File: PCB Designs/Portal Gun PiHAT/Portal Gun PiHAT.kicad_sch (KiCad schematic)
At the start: 26 parts, among them J1 GPIO, J2 SPARE_OUT_1, J3 SPARE_OUT_2, J4 NeoPixelFWD, J5 NeoPixelAFT, J6 5V Input, J7 PushButton2, J8 PushButton1, SW1 GPIO_SPARE_SW1, SW2 GPIO_SPARE_SW2, SW3 LED_PWR_SW, U1 CAT24C256

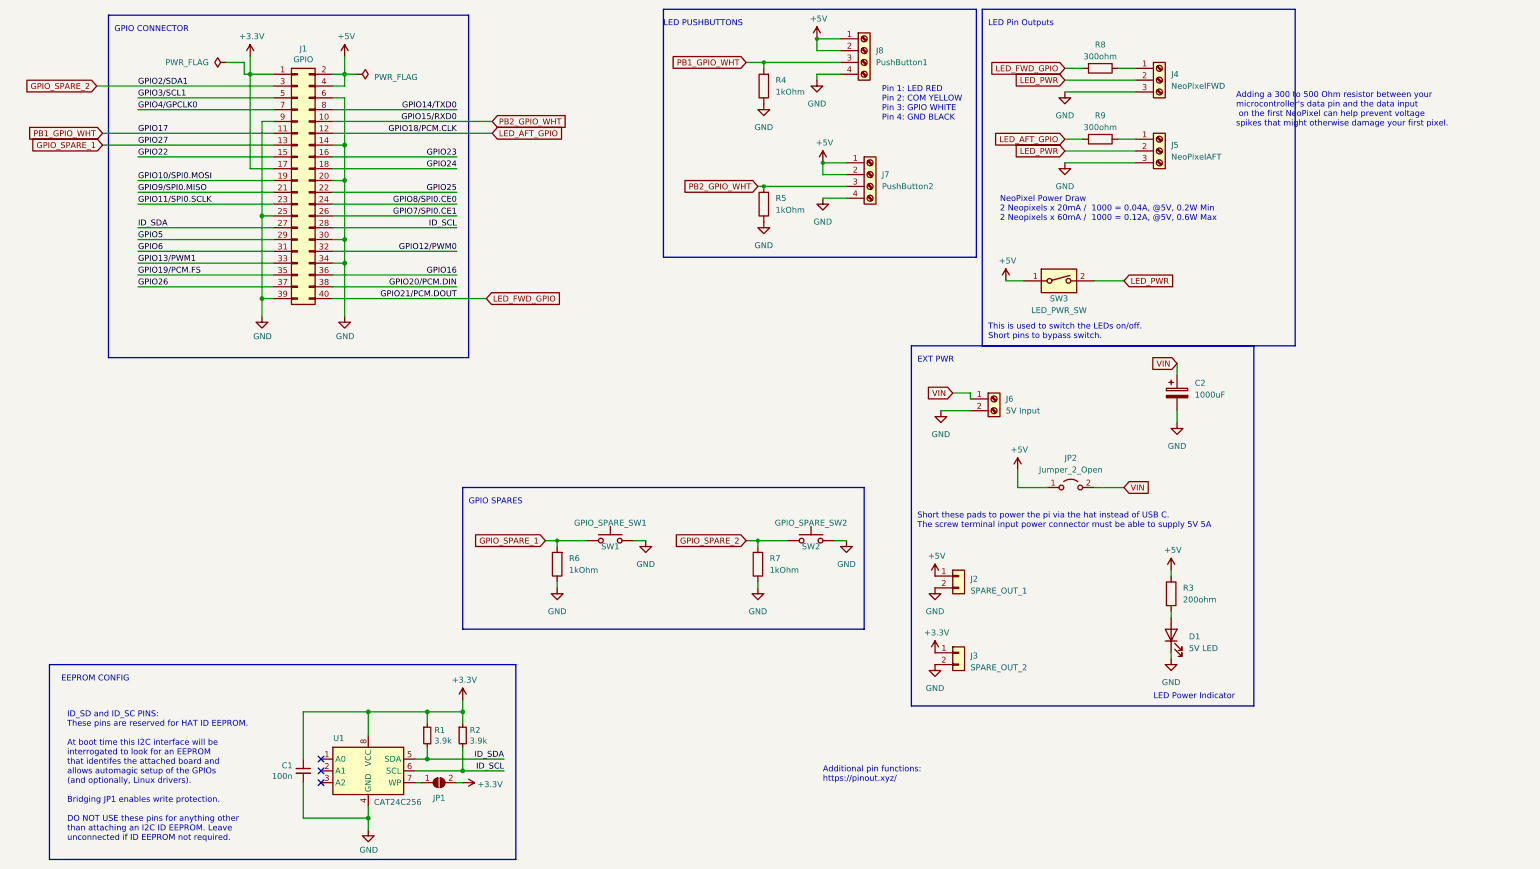
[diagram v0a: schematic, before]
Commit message: KiCad PCBs Finalized
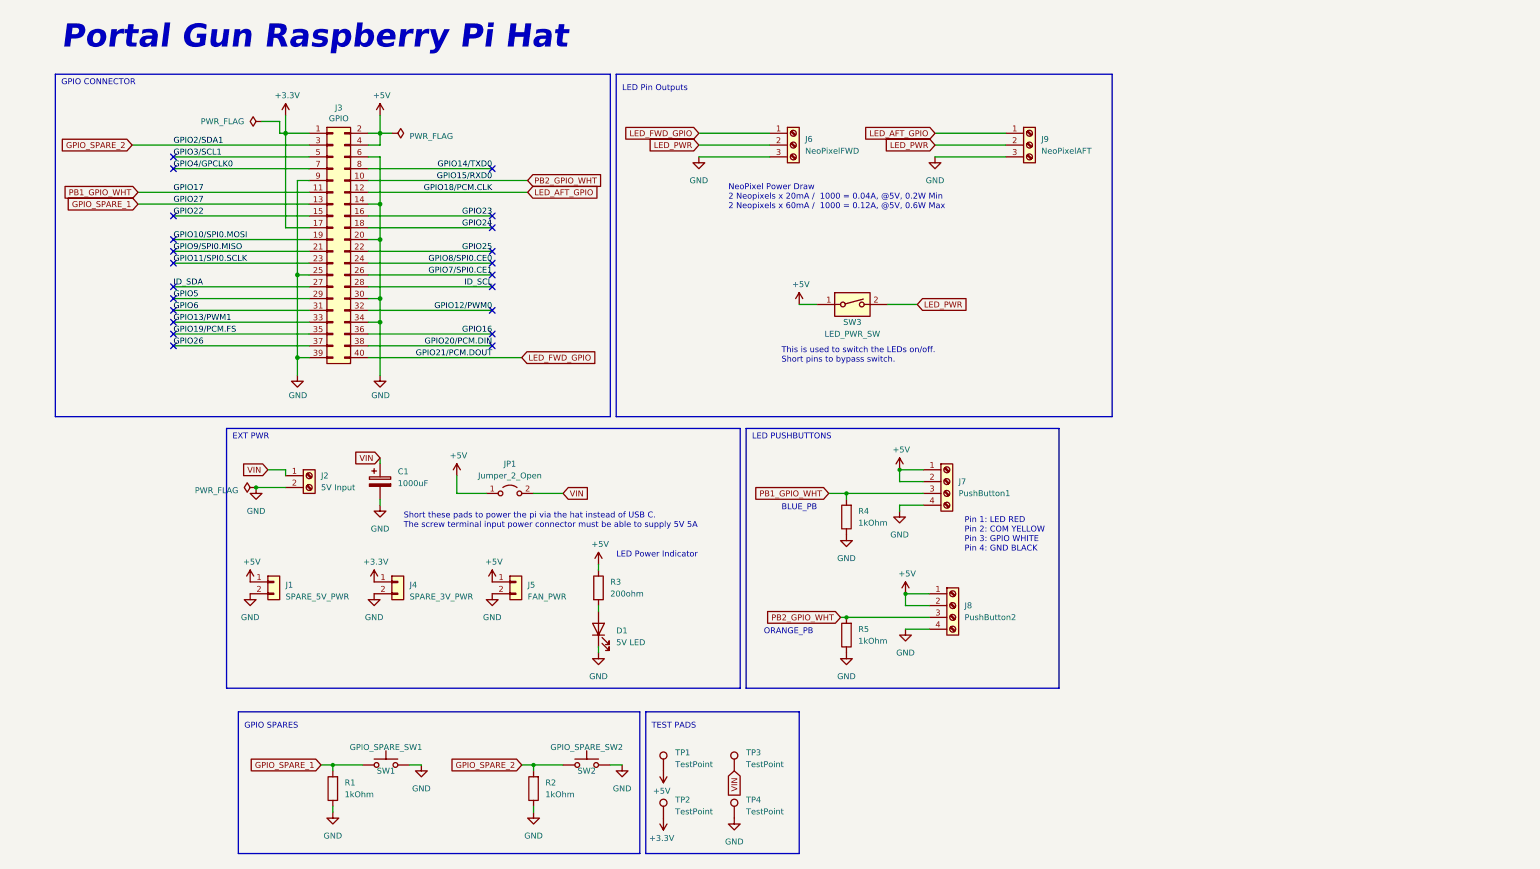
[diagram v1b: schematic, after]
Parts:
- removed C1: 100n, symbol Device:C_Small
- removed JP1: ID_WP, symbol Jumper:SolderJumper_2_Open
- removed R1, R2: 3.9k, symbol Device:R_Small
- removed R8, R9: 300ohm, symbol Device:R
- removed U1: CAT24C256, symbol Memory_EEPROM:CAT24C256
- added J5: FAN_PWR, Connector_PinHeader_2.54mm:PinHeader_1x02_P2.54mm_Vertical, symbol Connector_Generic:Conn_01x02
- added TP1, TP2, TP3, TP4: TestPoint, TestPoint:TestPoint_Pad_D1.0mm, symbol Connector:TestPoint
- C1: renamed from C2; footprint GrayFoxComponents:Horizontal Capacitor -> Capacitor_THT:C_Radial_D10.0mm_H16.0mm_P5.00mm
- D1: footprint (none) -> LED_THT:LED_D3.0mm
- J1: renamed from J2; value SPARE_OUT_1 -> SPARE_5V_PWR; footprint TerminalBlock_Phoenix:TerminalBlock_Phoenix_MKDS-1,5-2_1x02_P5.00mm_Horizontal -> Connector_PinHeader_2.54mm:PinHeader_1x02_P2.54mm_Vertical
- J2: renamed from J6; footprint (none) -> TerminalBlock_Phoenix:TerminalBlock_Phoenix_MKDS-1,5-2_1x02_P5.00mm_Horizontal
- J4: renamed from J3; value SPARE_OUT_2 -> SPARE_3V_PWR; footprint TerminalBlock_Phoenix:TerminalBlock_Phoenix_MKDS-1,5-2_1x02_P5.00mm_Horizontal -> Connector_PinHeader_2.54mm:PinHeader_1x02_P2.54mm_Vertical
- J6: renamed from J4; footprint (none) -> TerminalBlock_Phoenix:TerminalBlock_Phoenix_MKDS-1,5-3_1x03_P5.00mm_Horizontal
- J7: renamed from J8; footprint (none) -> TerminalBlock_Phoenix:TerminalBlock_Phoenix_MKDS-1,5-4_1x04_P5.00mm_Horizontal
- J8: renamed from J7; footprint (none) -> TerminalBlock_Phoenix:TerminalBlock_Phoenix_MKDS-1,5-4_1x04_P5.00mm_Horizontal
- J9: renamed from J5; footprint (none) -> TerminalBlock_Phoenix:TerminalBlock_Phoenix_MKDS-1,5-3_1x03_P5.00mm_Horizontal
- JP1: renamed from JP2; footprint (none) -> Jumper:SolderJumper-2_P1.3mm_Open_Pad1.0x1.5mm
- R1: renamed from R6; footprint (none) -> Resistor_SMD:R_1206_3216Metric_Pad1.30x1.75mm_HandSolder
- R2: renamed from R7; footprint (none) -> Resistor_SMD:R_1206_3216Metric_Pad1.30x1.75mm_HandSolder
- R3, R4, R5: footprint (none) -> Resistor_SMD:R_1206_3216Metric_Pad1.30x1.75mm_HandSolder
- renumbered J1 to J3
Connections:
- net +3V3: now also TP2.1
- net +5V: now also J5.1 (Pin_1), TP1.1
- net GND: now also J5.2 (Pin_2), TP4.1
- net LED_AFT_GPIO: now also J9.1 (Pin_1)
- net LED_FWD_GPIO: now also J6.1 (Pin_1)
- net VIN: now also TP3.1
- no-connect marks 3 -> 22
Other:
- note added: "BLUE_PB"
- note added: "ORANGE_PB"
- note added: "Portal Gun Raspberry Pi Hat"
- note added: "TEST PADS"
- note removed: "Adding a 300 to 500 Ohm resistor between your microcontroller's data pin and the data input on the first NeoPixel can help prevent voltage spikes that might otherwise damage your first pixel."
- note removed: "Additional pin functions: https://pinout.xyz/"
- note removed: "EEPROM CONFIG"
- note removed: "ID_SD and ID_SC PINS: These pins are reserved for HAT ID EEPROM. At boot time this I2C interface will be interrogated to look for an EEPROM that identifes the attached board and allows automagic setup of the GPIOs (and optionally, Linux drivers). Bridging JP1 enables write protection. DO NOT USE these pins for anything other than attaching an I2C ID EEPROM. Leave unconnected if ID EEPROM not requ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"
- company: (none) -> Ranil Ganlath
- title: (none) -> Portal Gun Raspberry Pi Hat PCB
- moved on the sheet: C1, D1, J1, J2, J3, J4, J6, J7, J8, J9, JP1, R1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
